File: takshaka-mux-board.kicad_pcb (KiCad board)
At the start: 2 copper layers, 31.6 x 24.2 mm, 12 parts, among them J1 Conn_01x01_Male, J2 Conn_01x01_Male, J3 Conn_02x08_Counter_Clockwise, J4 locked, J5 Conn_01x01_Male, J6 Conn_01x01_Male, U1 4051, U2 4051

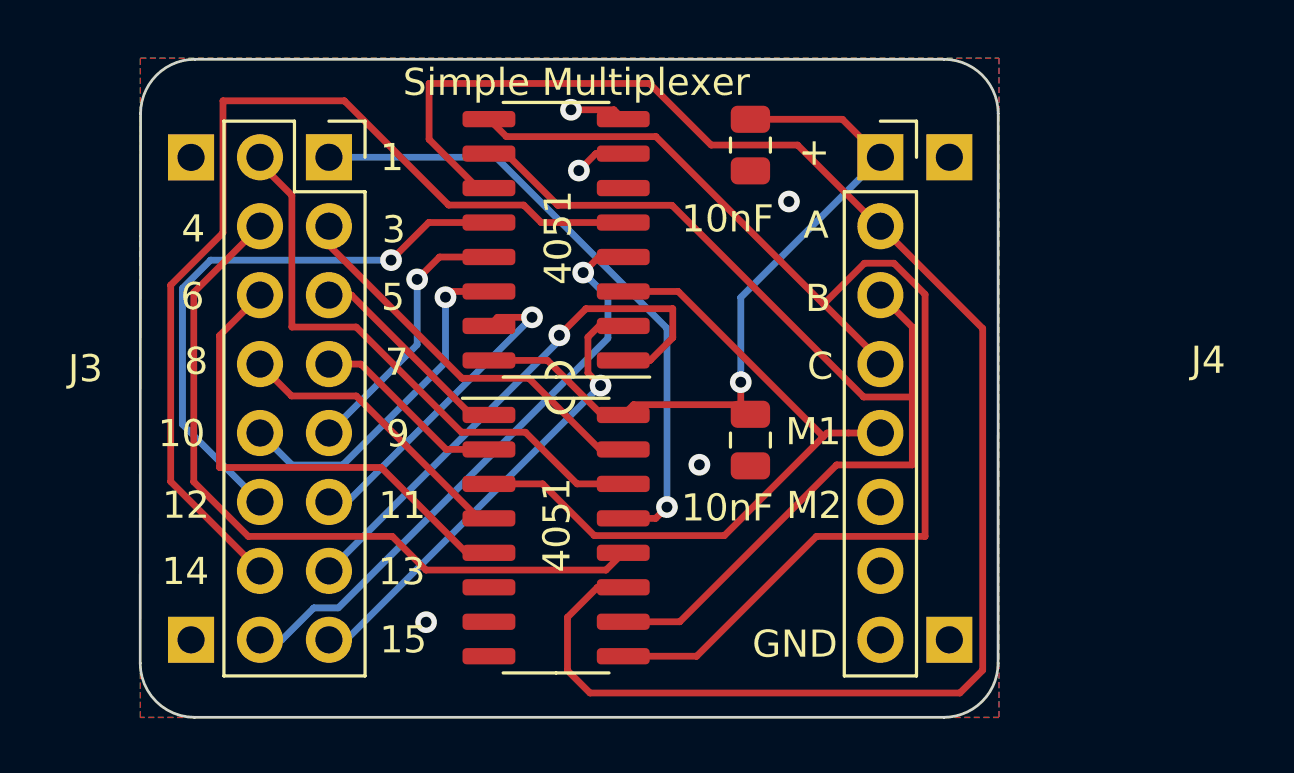
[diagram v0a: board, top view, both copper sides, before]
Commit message: rebuilt gerbers files.
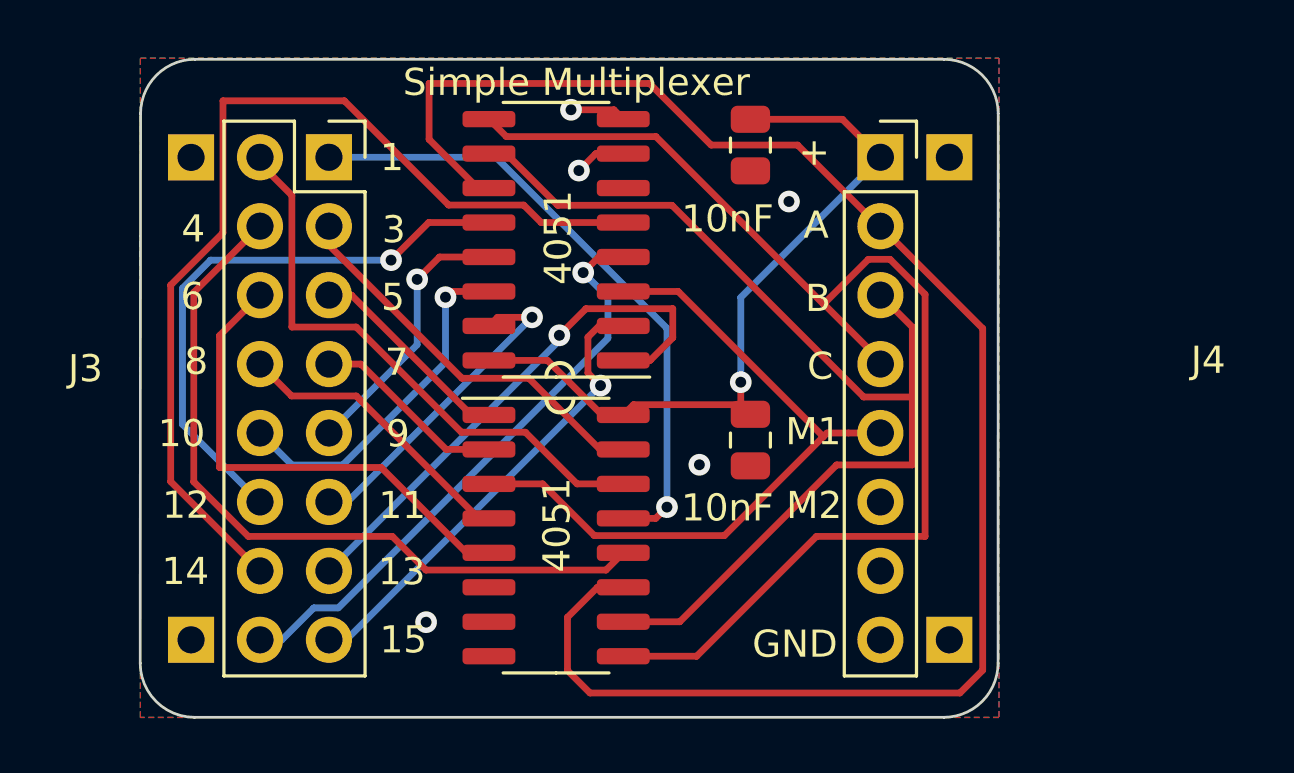
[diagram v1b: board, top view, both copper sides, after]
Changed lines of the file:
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@@
   (segment (start 251.9272 143.303) (end 250.133 143.303) (width 0.25) (layer "F.Cu") (net 8))
   (segment (start 248.6541 139.8844) (end 248.6744 139.8844) (width 0.25) (layer "F.Cu") (net 9))
+  (segment (start 250.3085 138.23) (end 248.6541 139.8844) (width 0.25) (layer "F.Cu") (net 9))
+  (segment (start 251.1051 138.23) (end 250.3085 138.23) (width 0.25) (layer "F.Cu") (net 9))
   (segment (start 252.3958 148.44) (end 252.3958 139.5207) (width 0.25) (layer "F.Cu") (net 9))
-  (segment (start 252.3958 139.5207) (end 251.2494 138.3743) (width 0.25) (layer "F.Cu") (net 9))
   (segment (start 248.6744 139.8844) (end 250.75 141.96) (width 0.25) (layer "F.Cu") (net 9))
+  (segment (start 250.75 141.96) (end 250.75 142.09) (width 0.25) (layer "F.Cu") (net 9))
+  (segment (start 248.6541 139.8844) (end 242.4787 133.709) (width 0.25) (layer "F.Cu") (net 9))
+  (segment (start 236.969 133.709) (end 236.325 133.065) (width 0.25) (layer "F.Cu") (net 9))
+  (segment (start 241.275 152.855) (end 243.9787 152.855) (width 0.25) (layer "F.Cu") (net 9))
+  (segment (start 248.3937 148.44) (end 252.3958 148.44) (width 0.25) (layer "F.Cu") (net 9))
+  (segment (start 242.4787 133.709) (end 236.969 133.709) (width 0.25) (layer "F.Cu") (net 9))
+  (segment (start 252.3958 139.5207) (end 251.1051 138.23) (width 0.25) (layer "F.Cu") (net 9))
   (segment (start 243.9787 152.855) (end 248.3937 148.44) (width 0.25) (layer "F.Cu") (net 9))
-  (segment (start 250.75 141.96) (end 250.75 142.09) (width 0.25) (layer "F.Cu") (net 9))
-  (segment (start 251.2494 138.3743) (end 250.1642 138.3743) (width 0.25) (layer "F.Cu") (net 9))
-  (segment (start 248.6541 139.8844) (end 242.4787 133.709) (width 0.25) (layer "F.Cu") (net 9))
-  (segment (start 241.275 152.855) (end 243.9787 152.855) (width 0.25) (layer "F.Cu") (net 9))
-  (segment (start 236.969 133.709) (end 236.325 133.065) (width 0.25) (layer "F.Cu") (net 9))
-  (segment (start 242.4787 133.709) (end 236.969 133.709) (width 0.25) (layer "F.Cu") (net 9))
-  (segment (start 248.3937 148.44) (end 252.3958 148.44) (width 0.25) (layer "F.Cu") (net 9))
-  (segment (start 250.1642 138.3743) (end 248.6541 139.8844) (width 0.25) (layer "F.Cu") (net 9))
   (segment (start 250.75 144.63) (end 249.5747 144.63) (width 0.25) (layer "F.Cu") (net 10))
   (segment (start 248.6477 144.7633) (end 248.781 144.63) (width 0.25) (layer "F.Cu") (net 10))
